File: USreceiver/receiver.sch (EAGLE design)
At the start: 10 parts, among them U1 LMP7712MM

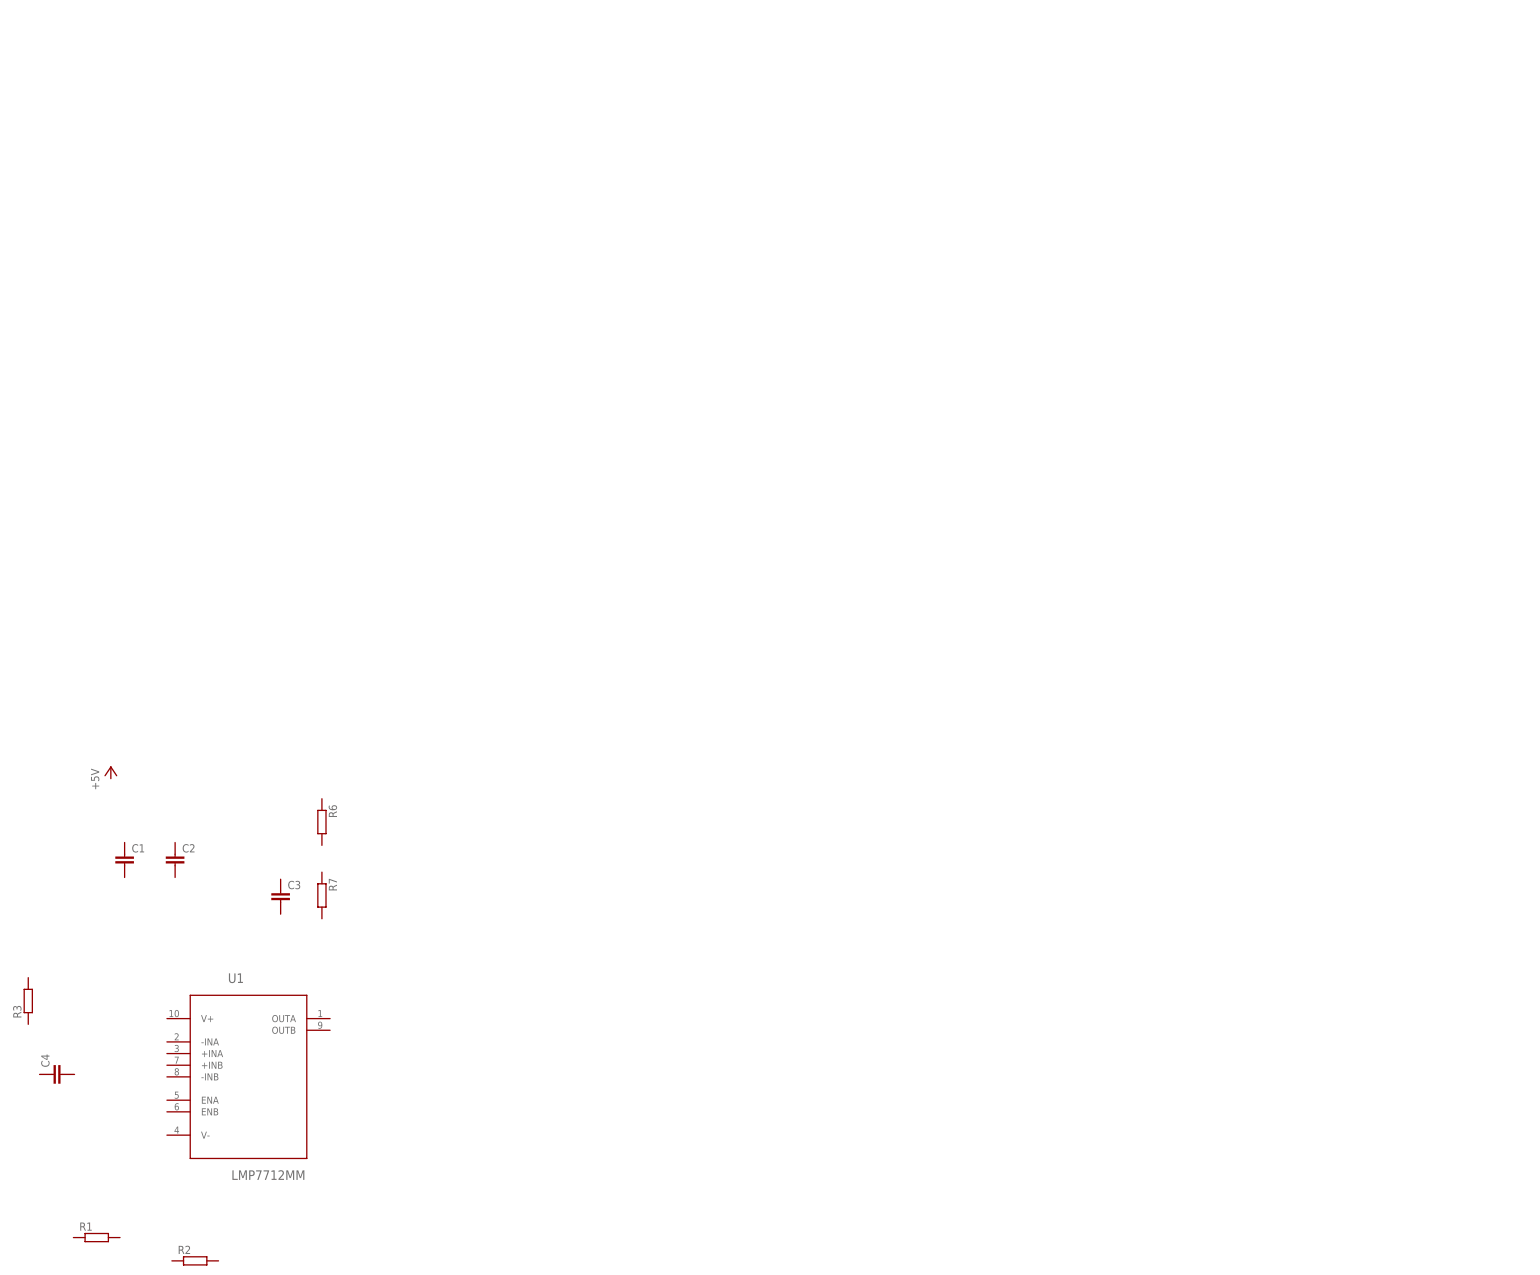
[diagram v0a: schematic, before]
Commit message: Schematic done. Board started. Library updated.
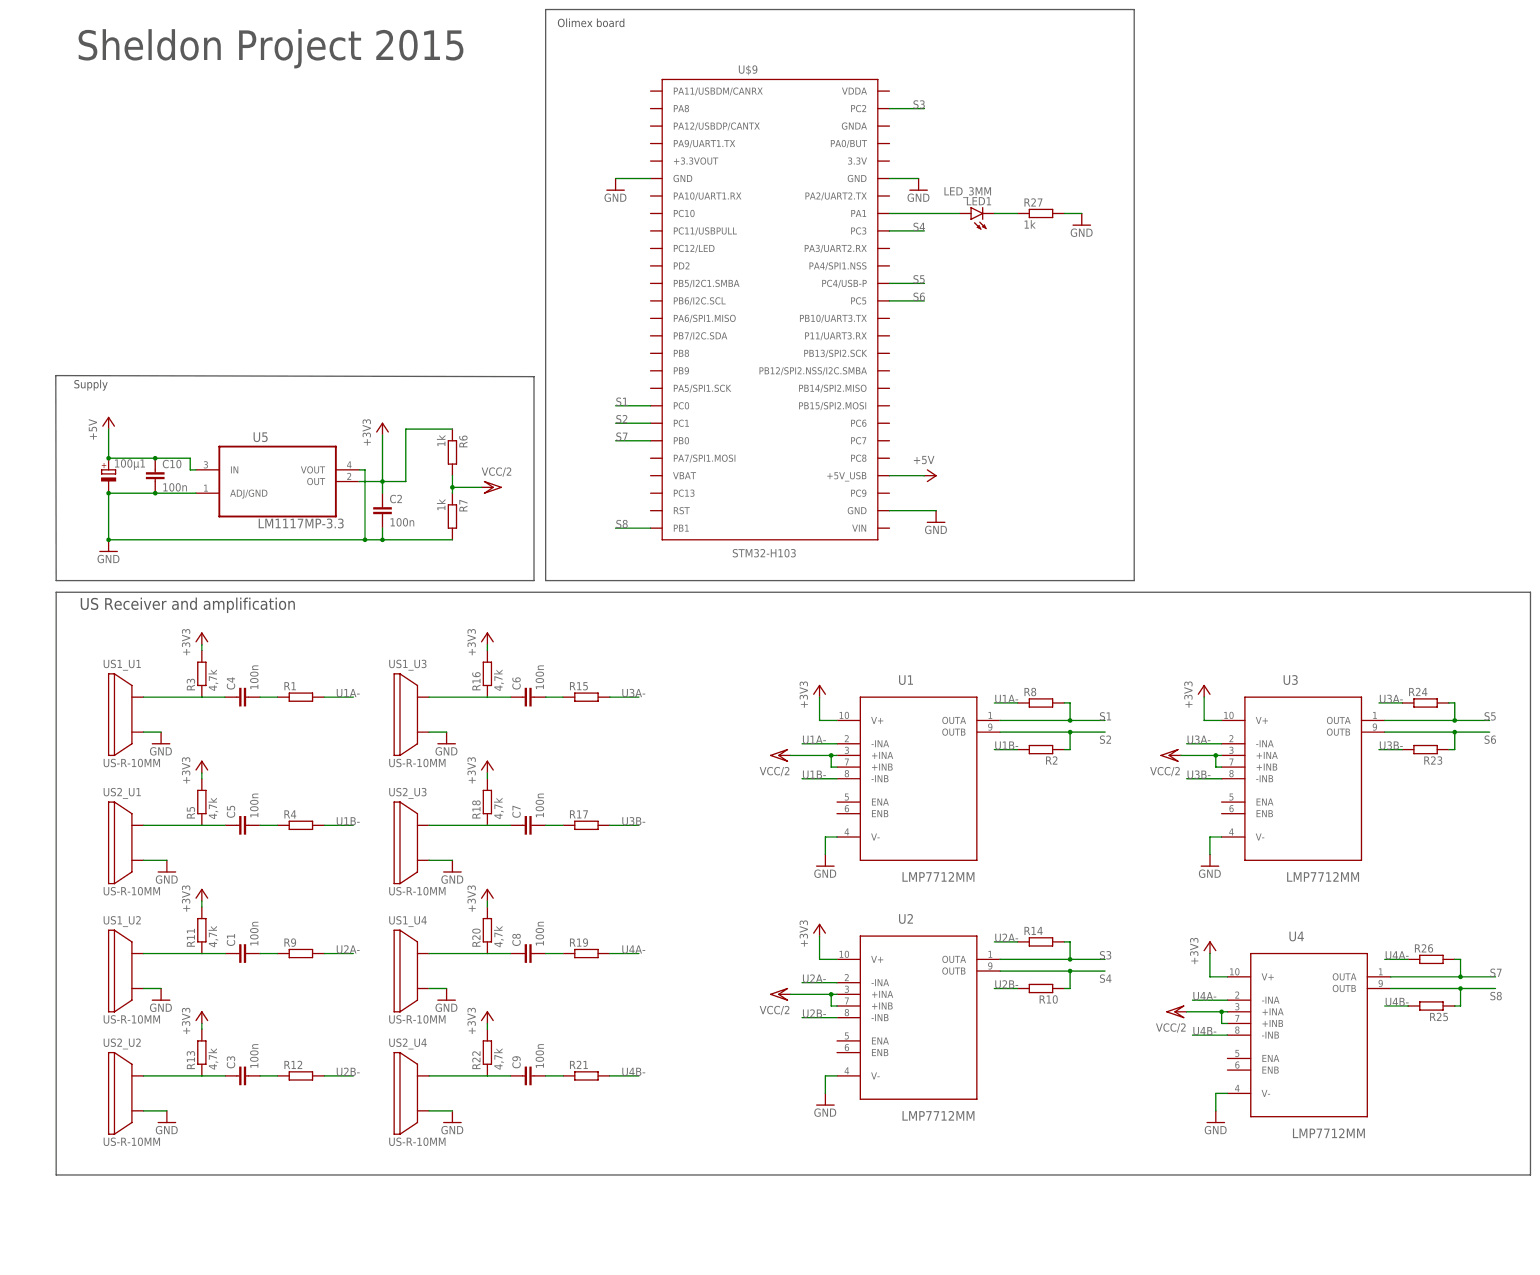
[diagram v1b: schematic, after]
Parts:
- added 100µ1: (no value), @Club_passif:CPOL_DIAM5MM
- added C10, C5, C6, C7, C8, C9: 100n, resistor:C-EUC0603
- added LED1: LED_3MM, @Club_passif:LED_3MM
- added R10, R12, R14, R15, R17, R19, R21, R23, R24, R25, R26, R4, R8, R9: (no value), resistor:R-EU_R0603
- added R11, R13, R16, R18, R20, R22, R5: 4,7k, resistor:R-EU_R0603
- added R27: 1k, resistor:R-EU_R0603
- added U$9: STM32-H103, libSheldonDrone:STM32-H103
- added U2, U3, U4: LMP7712MM, libSheldonDrone:LMP7712MM
- added U5: LM1117MP-3.3, libSheldonDrone:LM1117MP-3.3
- added US1_U1, US1_U2, US1_U3, US1_U4, US2_U1, US2_U2, US2_U3, US2_U4: US-R-10MM, libSheldonDrone:US-R-10MM
- C1, C2, C3, C4: value (none) -> 100n
- R3: value (none) -> 4,7k
- R6, R7: value (none) -> 1k
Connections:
- new net +3V3: C2.1, R11.2, R13.2, R16.2, R18.2, R20.2, R22.2, R3.2, R5.2, R6.1, U1.V+, U2.V+, U3.V+, U4.V+, U5.OUT
- new net +5V: 100µ1.P$1, C10.1, U$9.+5V_USB, U5.IN
- new net GND: 100µ1.P$2, C10.2, C2.2, R27.2, R7.2, U$9.GND@1, U$9.GND@2, U$9.GND@3, U1.V-, U2.V-, U3.V-, U4.V-, U5.ADJ/GND, U5.VOUT, US1_U1.P$2, US1_U2.P$2, US1_U3.P$2, US1_U4.P$2, US2_U1.P$2, US2_U2.P$2, US2_U3.P$2, US2_U4.P$2
- new net N$1: C1.1, R11.1, US1_U2.P$1
- new net N$10: C6.2, R15.1
- new net N$11: C7.1, R18.1, US2_U3.P$1
- new net N$12: C7.2, R17.1
- new net N$13: C8.1, R20.1, US1_U4.P$1
- new net N$14: C8.2, R19.1
- new net N$15: C9.1, R22.1, US2_U4.P$1
- new net N$16: C9.2, R21.1
- new net N$17: LED1.A, U$9.PA1
- new net N$18: LED1.C, R27.1
- new net N$2: C1.2, R9.1
- new net N$3: C4.1, R3.1, US1_U1.P$1
- new net N$4: C4.2, R1.1
- new net N$5: C5.1, R5.1, US2_U1.P$1
- new net N$6: C5.2, R4.1
- new net N$7: C3.1, R13.1, US2_U2.P$1
- new net N$8: C3.2, R12.1
- new net N$9: C6.1, R16.1, US1_U3.P$1
- new net S1: R8.2, U$9.PC0, U1.OUTA
- new net S2: R2.1, U$9.PC1, U1.OUTB
- new net S3: R14.2, U$9.PC2, U2.OUTA
- new net S4: R10.1, U$9.PC3, U2.OUTB
- new net S5: R24.2, U$9.PC4/USB-P, U3.OUTA
- new net S6: R23.1, U$9.PC5, U3.OUTB
- new net S7: R26.2, U$9.PB0, U4.OUTA
- new net S8: R25.1, U$9.PB1, U4.OUTB
- new net U1A-: R1.2, R8.1, U1.-INA
- new net U1B-: R2.2, R4.2, U1.-INB
- new net U2A-: R14.1, R9.2, U2.-INA
- new net U2B-: R10.2, R12.2, U2.-INB
- new net U3A-: R15.2, R24.1, U3.-INA
- new net U3B-: R17.2, R23.2, U3.-INB
- new net U4A-: R19.2, R26.1, U4.-INA
- new net U4B-: R21.2, R25.2, U4.-INB
- new net VCC/2: R6.2, R7.1, U1.+INA, U1.+INB, U2.+INA, U2.+INB, U3.+INA, U3.+INB, U4.+INA, U4.+INB
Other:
- note added: "Olimex board"
- note added: "Sheldon Project 2015"
- note added: "Supply"
- note added: "US Receiver and amplification"
- moved on the sheet: C1, C2, C3, C4, R1, R2, R3, R6, R7, U1
